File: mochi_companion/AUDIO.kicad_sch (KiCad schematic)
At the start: 10 parts, among them U3 MAX98357A

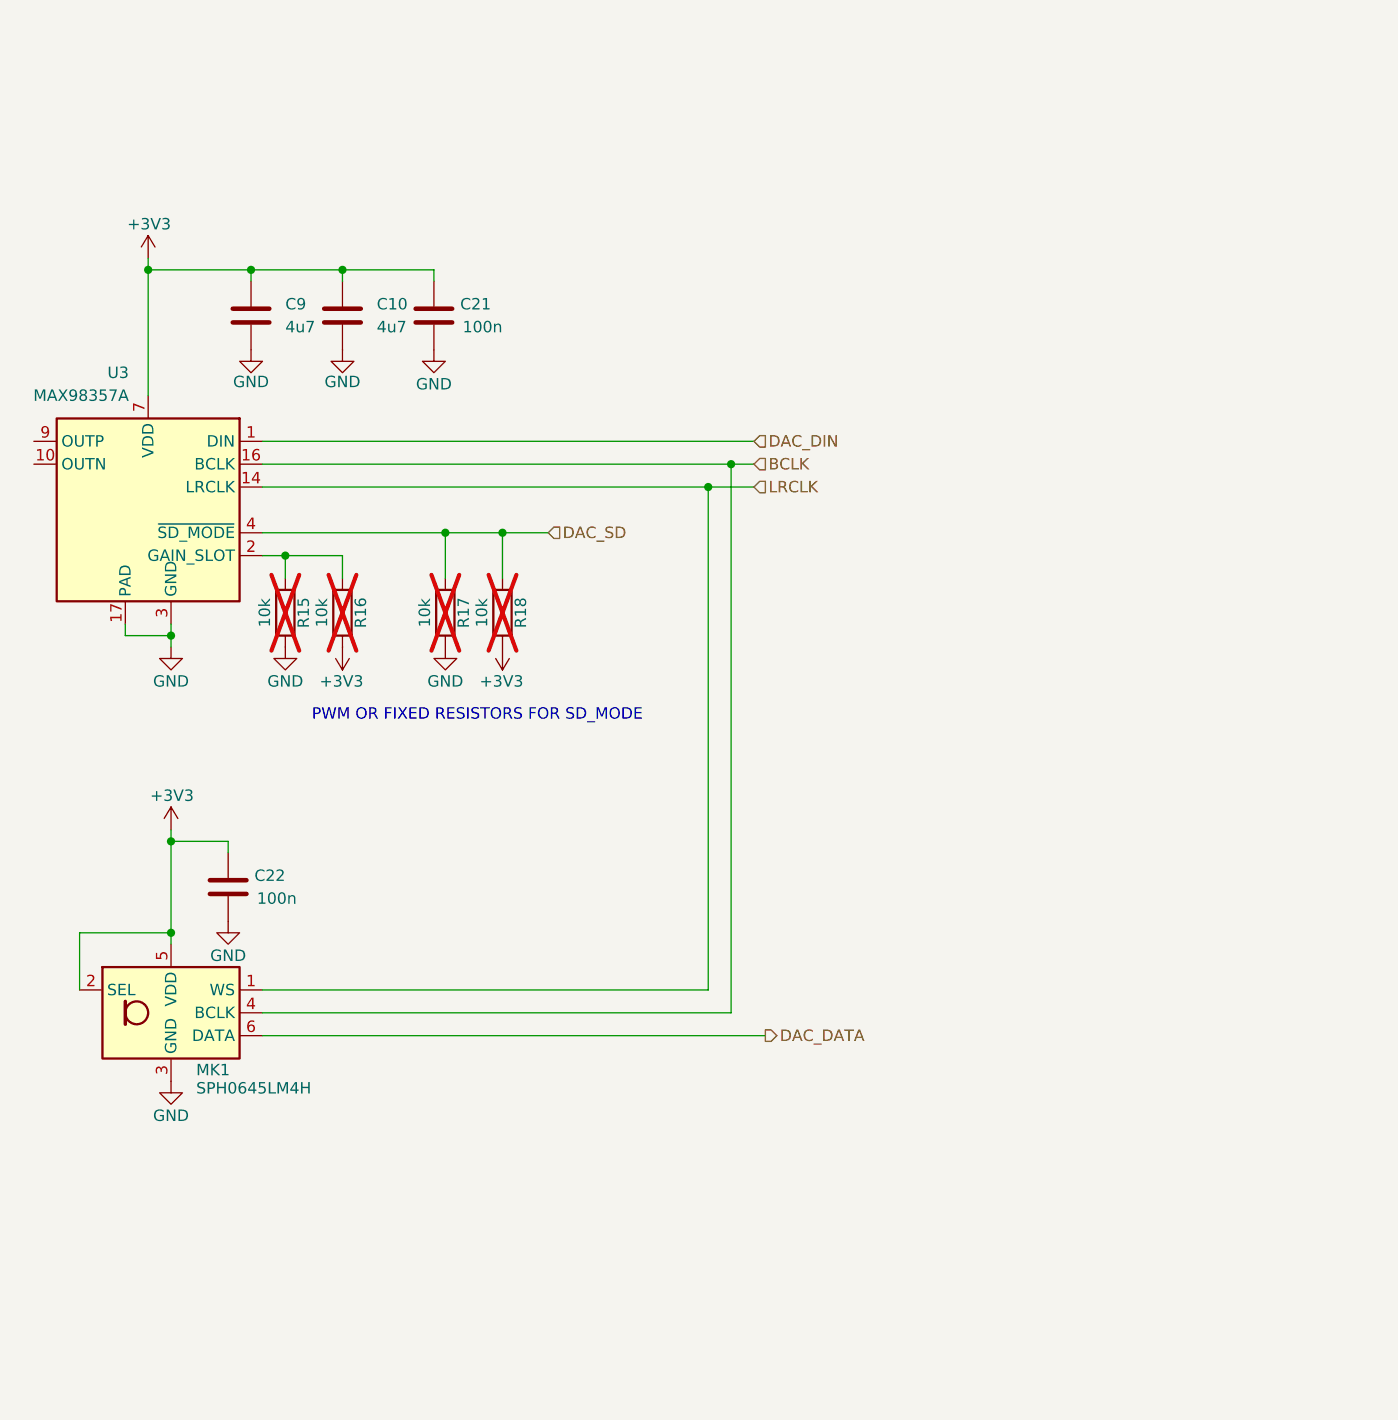
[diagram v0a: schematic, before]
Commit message: 250712_0041
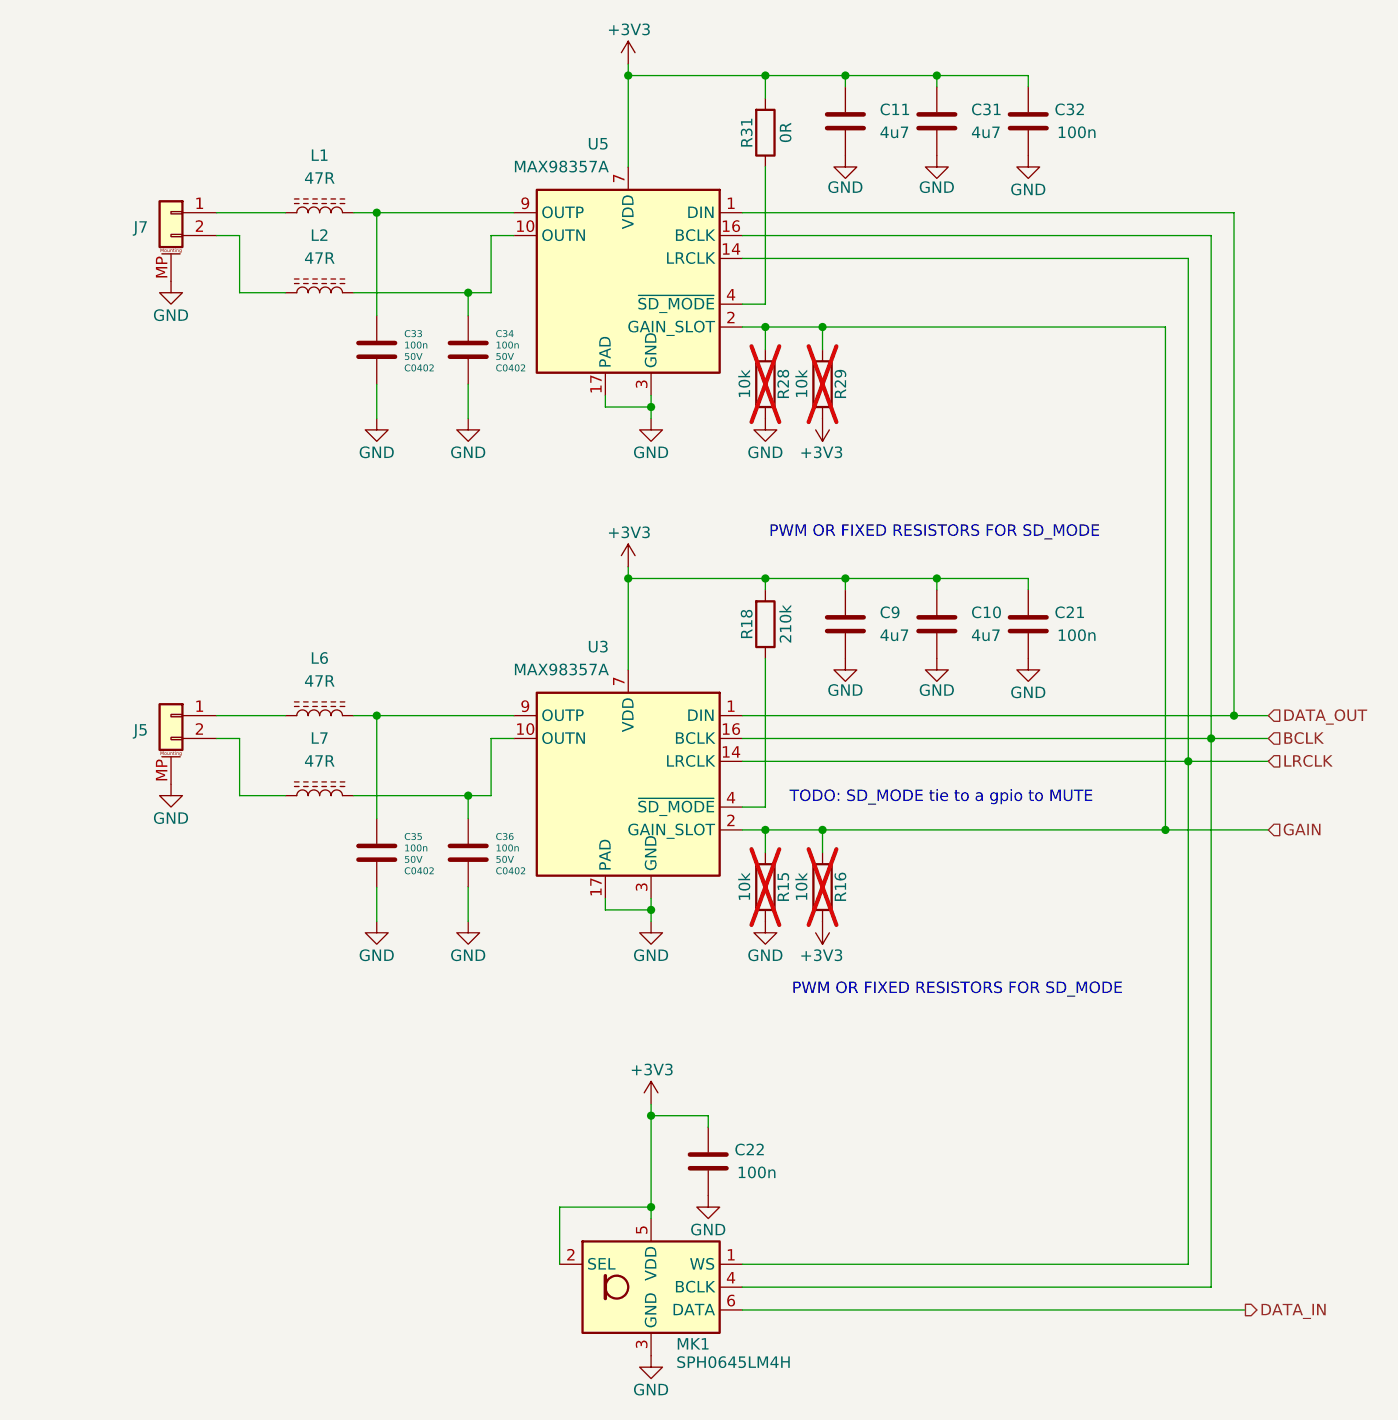
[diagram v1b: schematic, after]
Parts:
- removed R17: 10k, Resistor_SMD:R_0402_1005Metric, symbol Device:R
- added C11, C31: 4u7, Capacitor_SMD:C_0402_1005Metric, symbol Device:C
- added C32, C33, C34, C35, C36: 100n, Capacitor_SMD:C_0402_1005Metric, symbol Device:C
- added J5, J7: Conn_01x02_MountingPin, Connector_JST:JST_SHL_SM02B-SHLS-TF_1x02-1MP_P1.00mm_Horizontal, symbol Connector_Generic_MountingPin:Conn_01x02_MountingPin
- added L1, L2, L6, L7: 47R, Inductor_SMD:L_0402_1005Metric, symbol Device:L_Ferrite
- added R28, R29: 10k, Resistor_SMD:R_0402_1005Metric, symbol Device:R
- added R31: 0R, Resistor_SMD:R_0402_1005Metric, symbol Device:R
- added U5: MAX98357A, Package_DFN_QFN:TQFN-16-1EP_3x3mm_P0.5mm_EP1.23x1.23mm, symbol Audio:MAX98357A
- R18: value 10k -> 210k; now fitted
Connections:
- net +3V3: now also C11.1, C31.1, C32.1, R29.2, R31.2, U5.7 (VDD), U5.8 (VDD)
- net BCLK: now also U5.16 (BCLK)
- net GND: now also C11.2, C31.2, C32.2, C33.2, C34.2, C35.2, C36.2, J5.MP (MountPin), J7.MP (MountPin), R28.2, U5.11 (GND), U5.15 (GND), U5.17 (PAD), U5.3 (GND)
- net LRCLK: now also U5.14 (LRCLK)
- net GAIN: now reaches R15.1, R16.1, U3.2 (GAIN_SLOT)
- net GAIN: now also R28.1, R29.1, U5.2 (GAIN_SLOT)
- net at U3.10 (OUTN): now also C36.1, L7.2
- net at U3.9 (OUTP): now also C35.1, L6.2
- net DAC_DATA renamed DATA_IN
- net DAC_DIN renamed DATA_OUT
- net DATA_OUT: now also U5.1 (DIN)
- net DAC_SD: no longer names the net of R18.1, U3.4 (~{SD_MODE})
- new net: J5.1 (Pin_1), L6.1
- new net: J5.2 (Pin_2), L7.1
- new net: R31.1, U5.4 (~{SD_MODE})
- new net: C34.1, L2.2, U5.10 (OUTN)
- new net: C33.1, L1.2, U5.9 (OUTP)
- new net: J7.2 (Pin_2), L2.1
- new net: J7.1 (Pin_1), L1.1
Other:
- note added: "TODO: SD_MODE tie to a gpio to MUTE"
- moved on the sheet: C10, C21, C22, C9, MK1, R15, R16, U3
